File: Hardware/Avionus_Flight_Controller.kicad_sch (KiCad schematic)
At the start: 0 parts

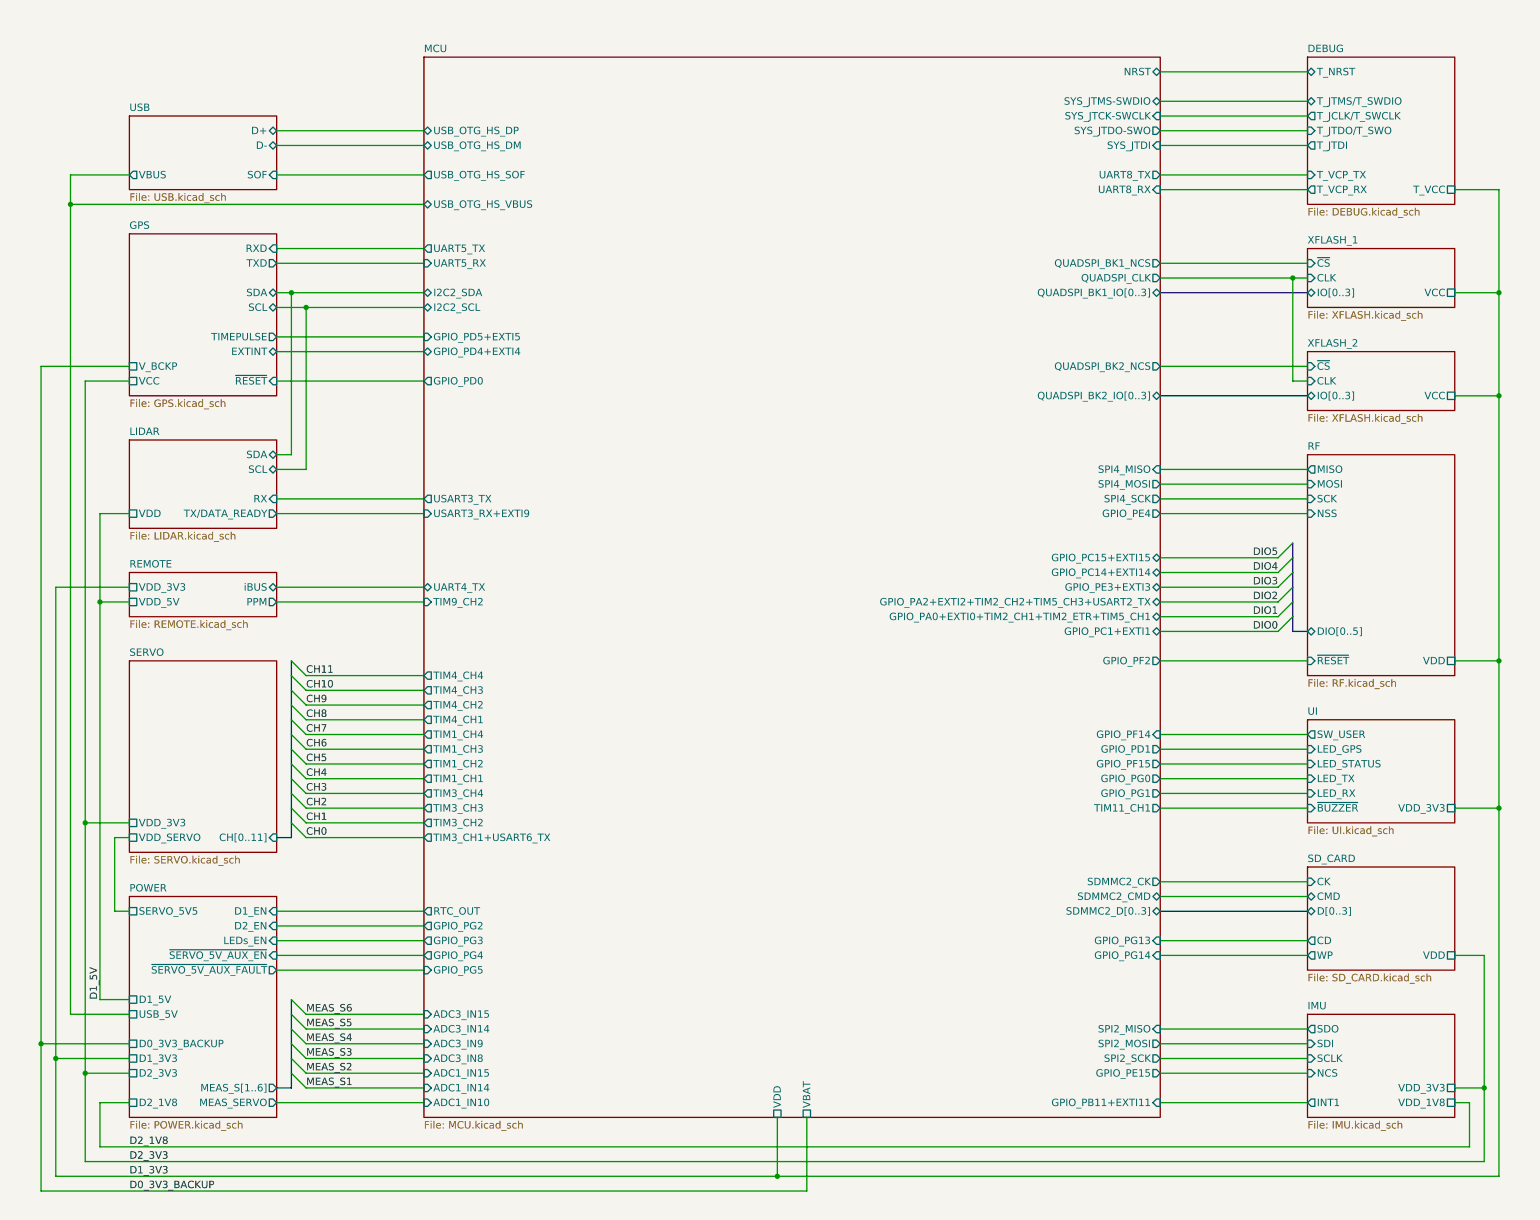
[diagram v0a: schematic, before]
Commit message: Checkpoint
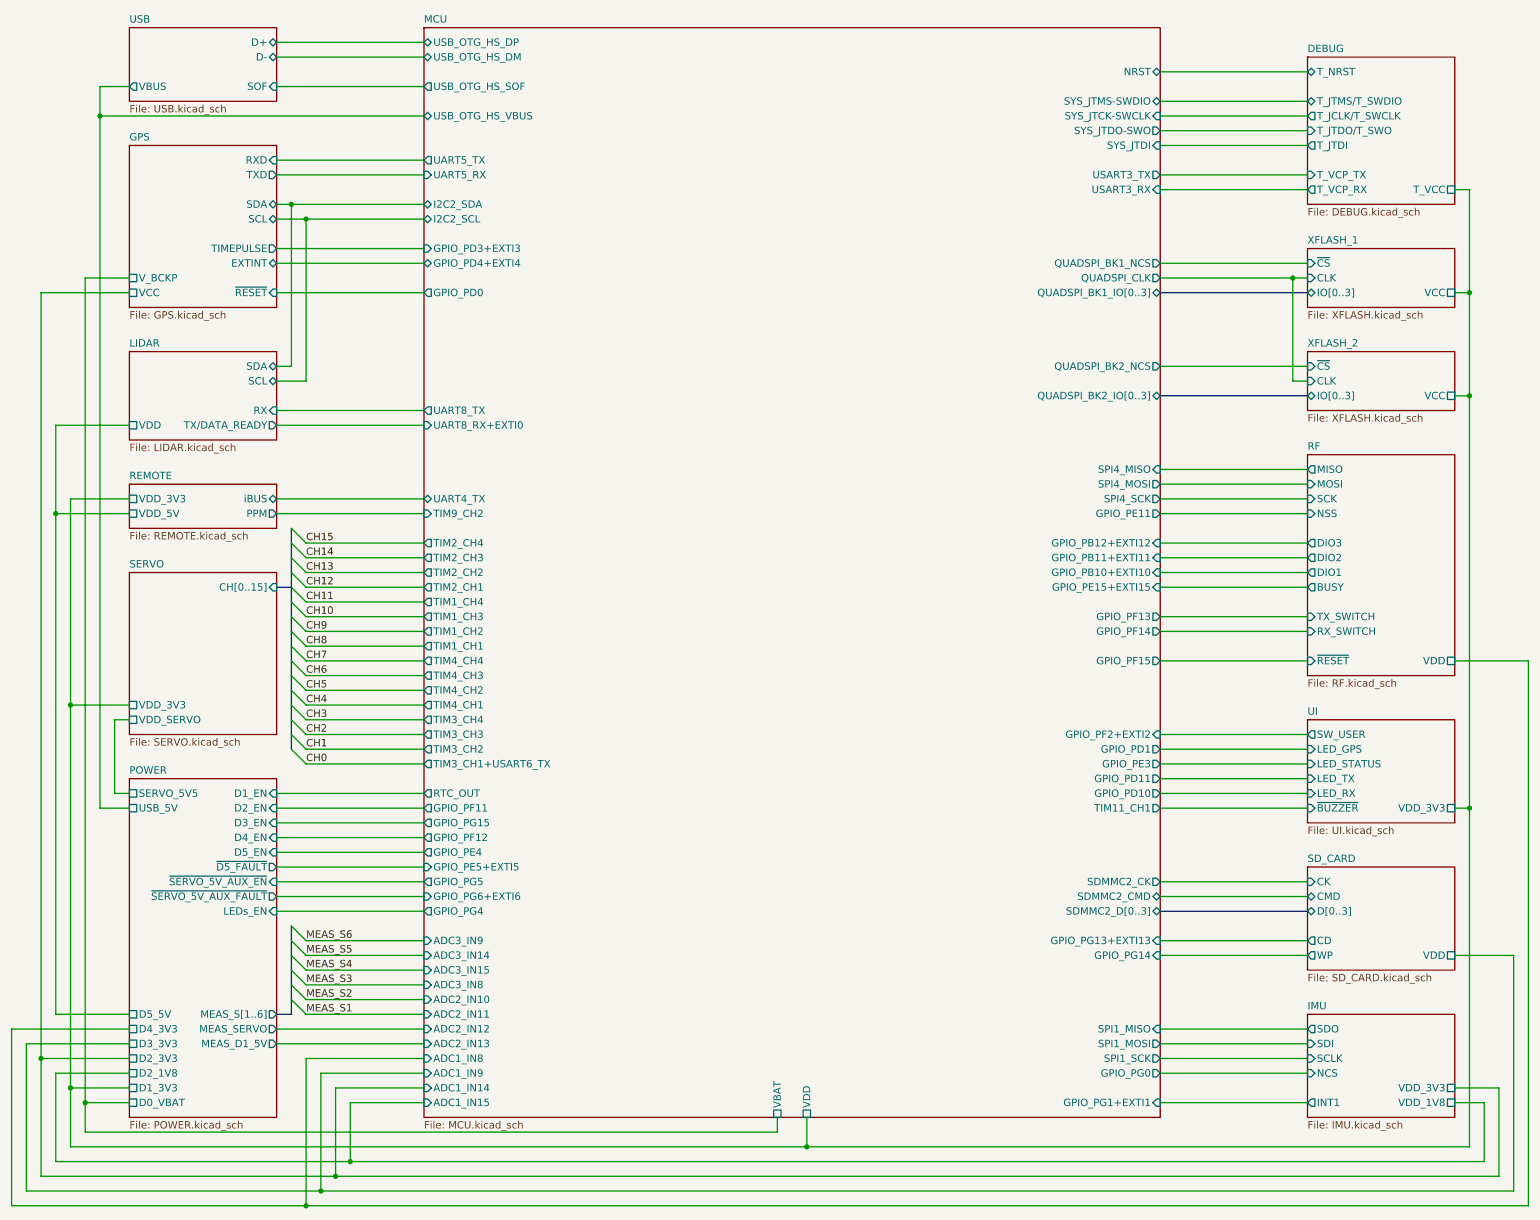
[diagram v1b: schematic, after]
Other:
- sheet MCU ports: added ADC1_IN8, ADC1_IN9, ADC2_IN10, ADC2_IN11, ADC2_IN12, ADC2_IN13, GPIO_PB10+EXTI10, GPIO_PB12+EXTI12, GPIO_PD10, GPIO_PD11, GPIO_PD3+EXTI3, GPIO_PE11, GPIO_PE15+EXTI15, GPIO_PE3, GPIO_PE5+EXTI5, GPIO_PF11, GPIO_PF12, GPIO_PF13, GPIO_PF2+EXTI2, GPIO_PG1+EXTI1, GPIO_PG13+EXTI13, GPIO_PG15, GPIO_PG6+EXTI6, SPI1_MISO, SPI1_MOSI, SPI1_SCK, TIM2_CH1, TIM2_CH2, TIM2_CH3, TIM2_CH4, UART8_RX+EXTI0, USART3_RX; removed ADC1_IN10, GPIO_PA0+EXTI0+TIM2_CH1+TIM2_ETR+TIM5_CH1, GPIO_PA2+EXTI2+TIM2_CH2+TIM5_CH3+USART2_TX, GPIO_PC1+EXTI1, GPIO_PC14+EXTI14, GPIO_PC15+EXTI15, GPIO_PD5+EXTI5, GPIO_PE15, GPIO_PE3+EXTI3, GPIO_PF2, GPIO_PG1, GPIO_PG13, GPIO_PG2, GPIO_PG3, SPI2_MISO, SPI2_MOSI, SPI2_SCK, UART8_RX, USART3_RX+EXTI9
- sheet POWER ports: added D0_VBAT, D3_3V3, D3_EN, D4_3V3, D4_EN, D5_5V, D5_EN, MEAS_D1_5V, ~{D5_FAULT}; removed D0_3V3_BACKUP, D1_5V
- sheet RF ports: added BUSY, DIO1, DIO2, DIO3, RX_SWITCH, TX_SWITCH; removed DIO[0..5]
- sheet SERVO ports: added CH[0..15]; removed CH[0..11]
